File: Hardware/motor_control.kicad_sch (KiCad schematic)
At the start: 5 parts, among them J5 Conn_01x02_Male, U5 DRV8212P

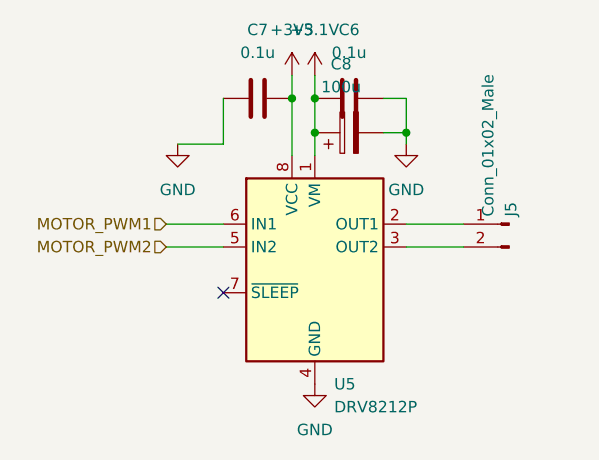
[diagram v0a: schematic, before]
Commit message: Fixed power
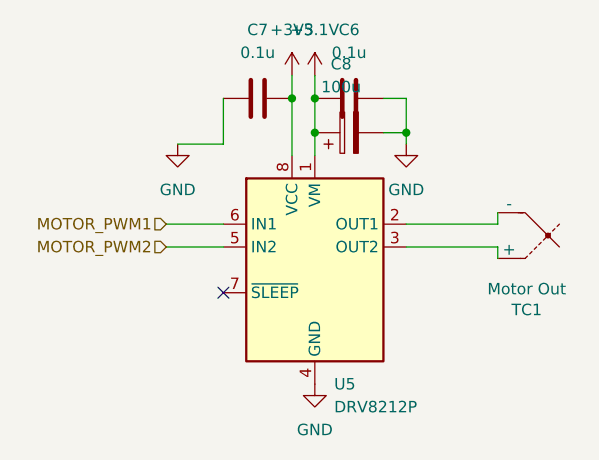
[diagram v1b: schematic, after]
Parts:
- removed J5: Conn_01x02_Male, TerminalBlock_Phoenix:TerminalBlock_Phoenix_PT-1,5-2-3.5-H_1x02_P3.50mm_Horizontal, symbol Connector:Conn_01x02_Male
- added TC1: Motor Out, Connector_Molex:Molex_Nano-Fit_105313-xx02_1x02_P2.50mm_Horizontal, symbol Device:Thermocouple
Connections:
- net at U5.2 (OUT1): now also TC1.2 (-)
- net at U5.3 (OUT2): now also TC1.1 (+)
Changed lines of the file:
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@@
 	(wire
 		(pts
-			(xy 190.5 64.77) (xy 196.85 64.77)
+			(xy 200.66 64.77) (xy 200.66 63.5)
+		)
+		(stroke
+			(width 0)
+			(type default)
+		)
+	)
+	(wire
+		(pts
+			(xy 190.5 64.77) (xy 200.66 64.77)
 		)
 		(stroke
@@
 	(wire
 		(pts
+			(xy 200.66 67.31) (xy 200.66 68.58)
+		)
+		(stroke
+			(width 0)
+			(type default)
+		)
+	)
+	(wire
+		(pts
 			(xy 163.83 64.77) (xy 170.18 64.77)
 		)
@@
 	(wire
 		(pts
-			(xy 190.5 67.31) (xy 196.85 67.31)
+			(xy 190.5 67.31) (xy 200.66 67.31)
 		)
 		(stroke
@@
 			)
 			(justify right)
+		)
+	)
+	(symbol
+		(lib_id "Device:Thermocouple")
+		(at 203.2 66.04 180)
+		(unit 1)
+		(exclude_from_sim no)
+		(in_bom yes)
+		(on_board yes)
+		(dnp no)
+		(property "Reference" "TC1"
+			(at 203.8858 74.295 0)
+			(effects
+				(font
+					(size 1.27 1.27)
+				)
+			)
+		)
+		(property "Value" "Motor Out"
+			(at 203.8858 71.9836 0)
+			(effects
+				(font
+					(size 1.27 1.27)
+				)
+			)
+		)
+		(property "Footprint" "Connector_Molex:Molex_Nano-Fit_105313-xx02_1x02_P2.50mm_Horizontal"
+			(at 217.805 67.31 0)
+			(effects
+				(font
+					(size 1.27 1.27)
+				)
+				(hide yes)
+			)
+		)
+		(property "Datasheet" "~"
+			(at 217.805 67.31 0)
+			(effects
+				(font
+					(size 1.27 1.27)
+				)
+				(hide yes)
+			)
+		)
+		(property "Description" ""
+			(at 203.2 66.04 0)
+			(effects
+				(font
+					(size 1.27 1.27)
+				)
+				(hide yes)
+			)
+		)
+		(pin "1"
+		)
+		(pin "2"
+		)
+		(instances
+			(project "Ricardo-Cappy"
+				(path "/e4035b22-64c9-4a42-9837-ade8aec3882f/4569c248-8a44-4db3-b2ae-2ad0733be142"
+					(reference "TC1")
+					(unit 1)
+				)
+			)
 		)
 	)
@@
 					(unit 1)
 				)
-			)
-		)
-	)
-	(symbol
-		(lib_id "Connector:Conn_01x02_Male")
-		(at 201.93 64.77 0)
-		(mirror y)
-		(unit 1)
-		(exclude_from_sim no)
-		(in_bom yes)
-		(on_board yes)
-		(dnp no)
-		(property "Reference" "J5"
-			(at 202.1297 63.9318 90)
-			(effects
-				(font
-					(size 1.27 1.27)
-				)
-				(justify left)
-			)
-		)
-		(property "Value" "Conn_01x02_Male"
-			(at 199.5928 63.9318 90)
-			(effects
-				(font
-					(size 1.27 1.27)
-				)
-				(justify left)
-			)
-		)
-		(property "Footprint" "TerminalBlock_Phoenix:TerminalBlock_Phoenix_PT-1,5-2-3.5-H_1x02_P3.50mm_Horizontal"
-			(at 201.93 64.77 0)
-			(effects
-				(font
-					(size 1.27 1.27)
-				)
-				(hide yes)
-			)
-		)
-		(property "Datasheet" "~"
-			(at 201.93 64.77 0)
-			(effects
-				(font
-					(size 1.27 1.27)
-				)
-				(hide yes)
-			)
-		)
-		(property "Description" ""
-			(at 201.93 64.77 0)
-			(effects
-				(font
-					(size 1.27 1.27)
-				)
-				(hide yes)
-			)
-		)
-		(pin "1"
-		)
-		(pin "2"
-		)
-		(instances
-			(project "Ricardo-Cappy"
-				(path "/e4035b22-64c9-4a42-9837-ade8aec3882f/4569c248-8a44-4db3-b2ae-2ad0733be142"
-					(reference "J5")
-					(unit 1)
-				)
